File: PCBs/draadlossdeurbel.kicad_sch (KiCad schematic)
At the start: 15 parts, among them J1 AudioJack4_Ground, Q1 BC161, U1 WeMos_D1_mini, U2 LM386, U3 74HC595, U4 SN76489

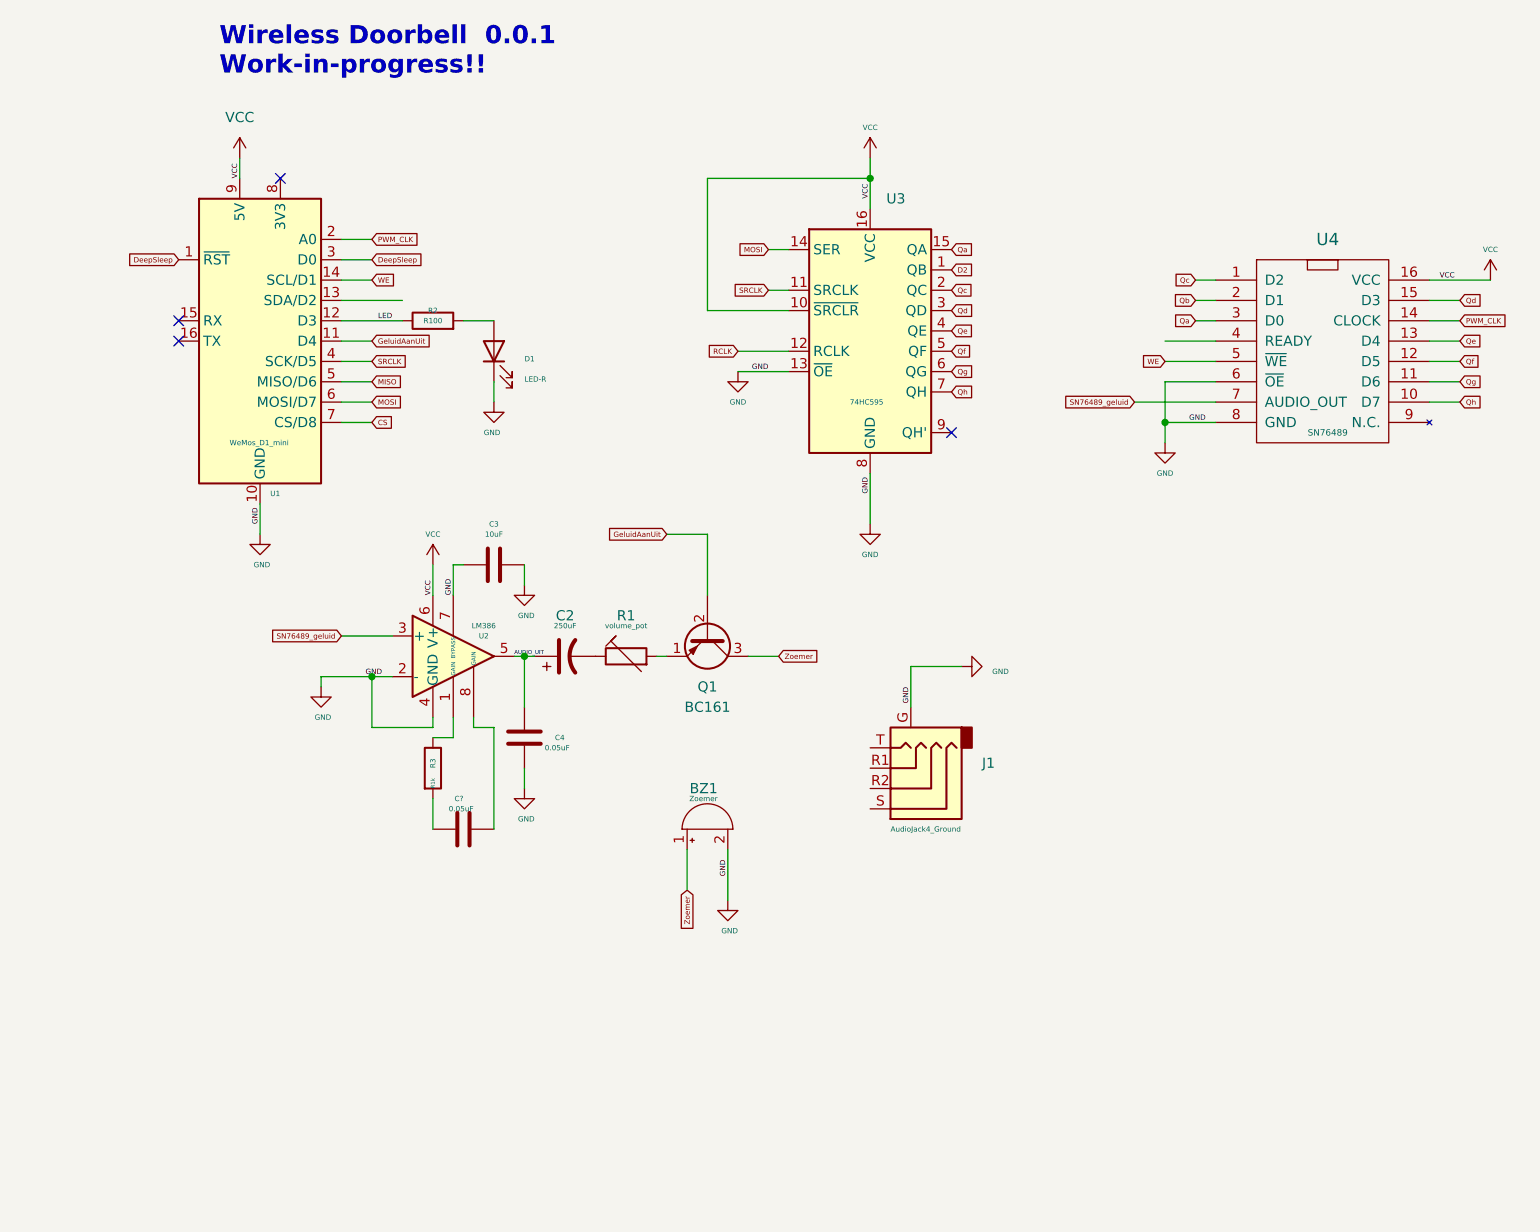
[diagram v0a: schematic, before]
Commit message: bijgewerkt
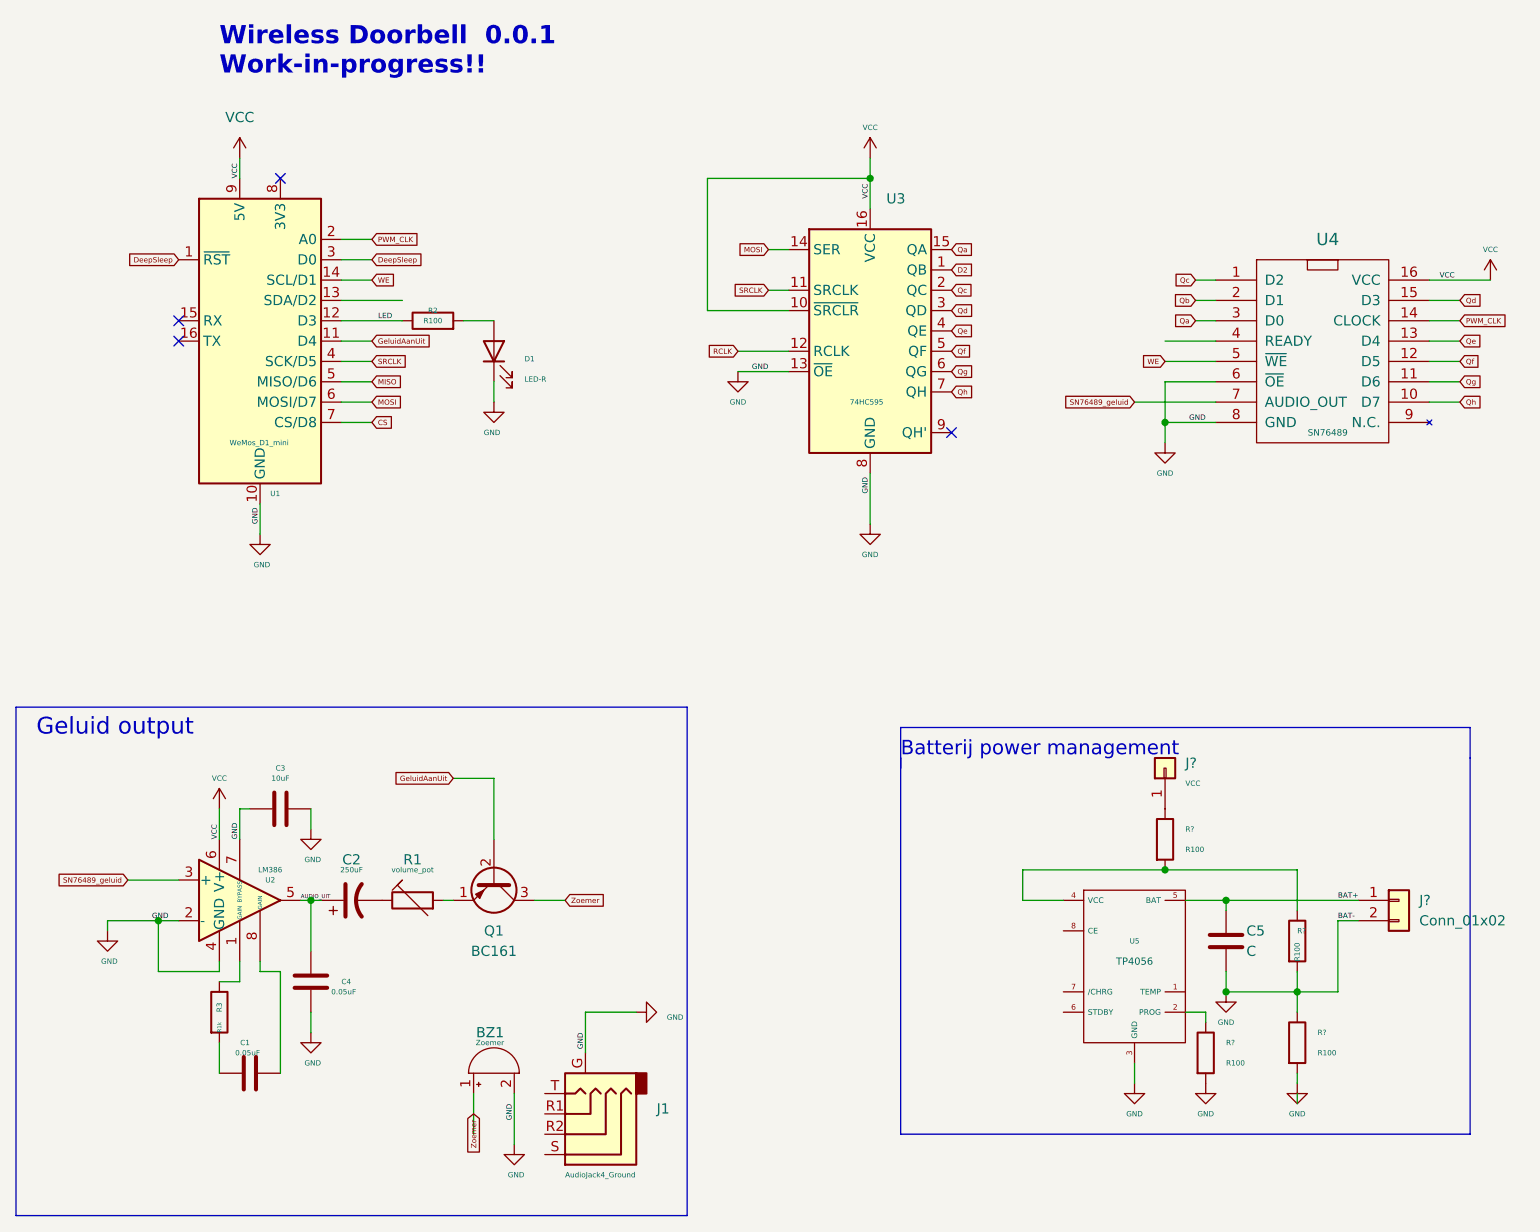
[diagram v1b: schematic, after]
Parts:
- added C5: C, symbol Device:C
- added J?: VCC, symbol Connector_Generic:Conn_01x01
- added J?: Conn_01x02, symbol Connector_Generic:Conn_01x02
- added R? (x4): R100, symbol Device:R
- added U5: TP4056, symbol EasyLab4Kids:TP4056
- gave numbers to parts that had none: 1
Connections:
- net GND: now also C5.2, J?.2 (Pin_2), R?.1, R?.2, R?.2, R?.2, U5.3 (GND)
- new net: R?.1, U5.2 (PROG)
- new net: R?.1, R?.2, U5.4 (VCC)
- new net: J?.1 (Pin_1), R?.1
- new net BAT+: C5.1, J?.1 (Pin_1), U5.5 (BAT)
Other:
- note added: "Batterij power management"
- note added: "Geluid output"
- moved on the sheet: BZ1, C1, C2, C3, C4, J1, Q1, R1, R3, U2
